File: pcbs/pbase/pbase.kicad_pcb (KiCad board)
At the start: 2 copper layers, 152.9 x 129.5 mm, 40 parts, among them J1 SD_Card, J2 Conn_01x04, J3 Conn_01x04, U1 LPCXpresso_LPC1769_revB, U2 acc_mpu9250_board, U3 GPS_EM506

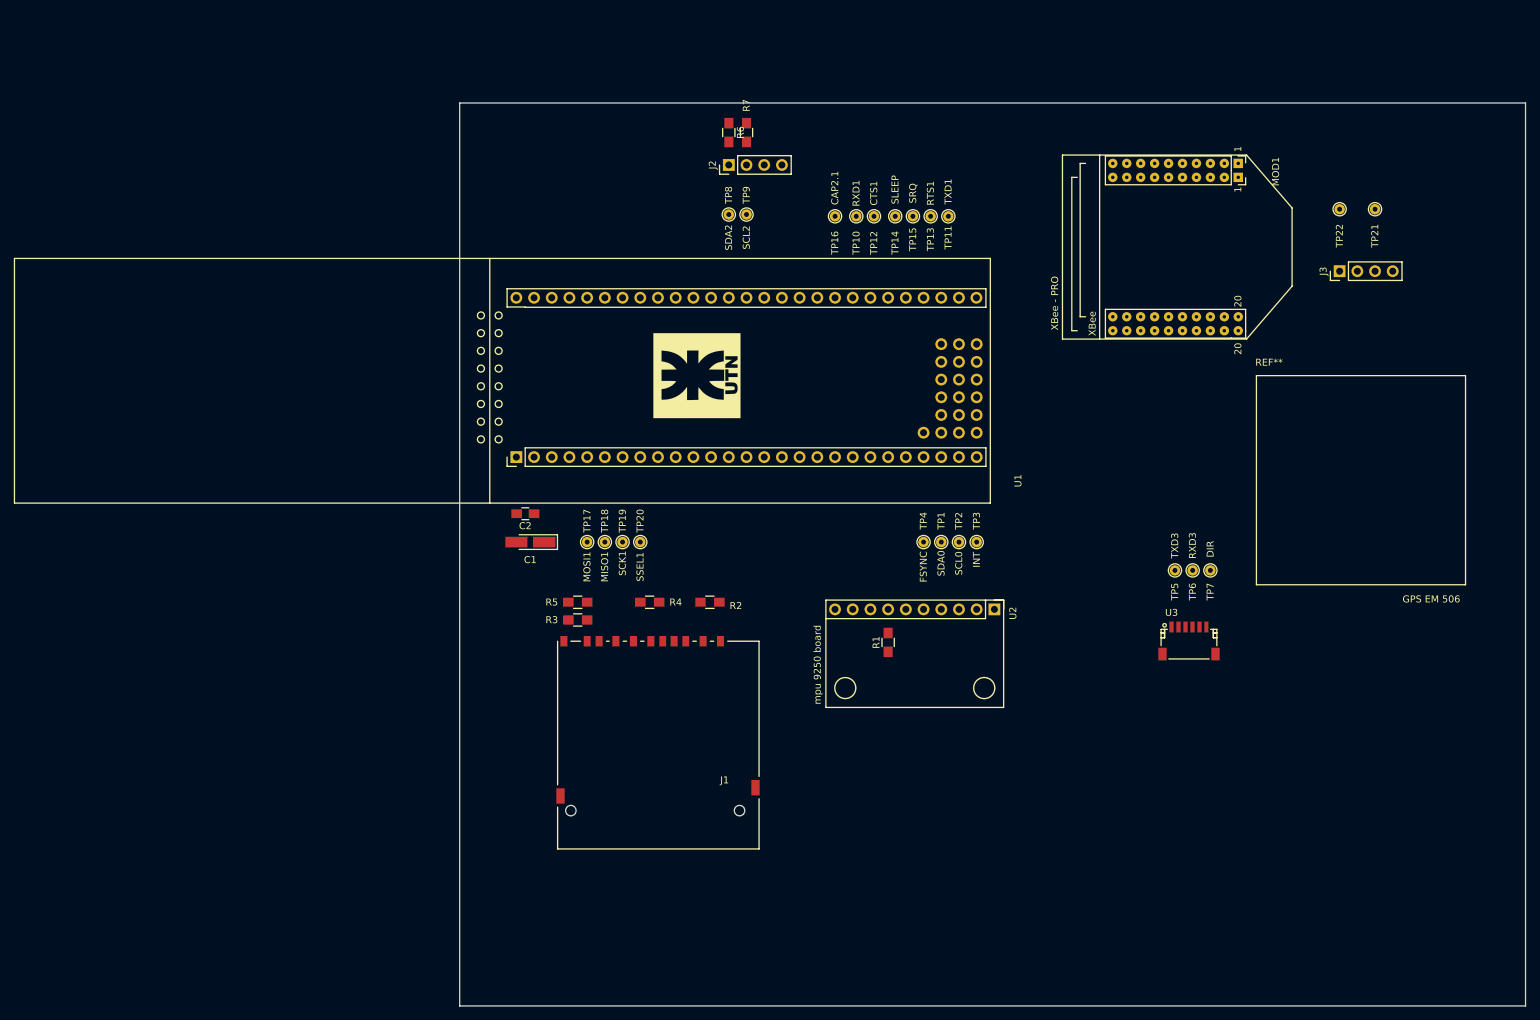
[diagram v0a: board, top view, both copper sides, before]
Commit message: PCB PLACING V1
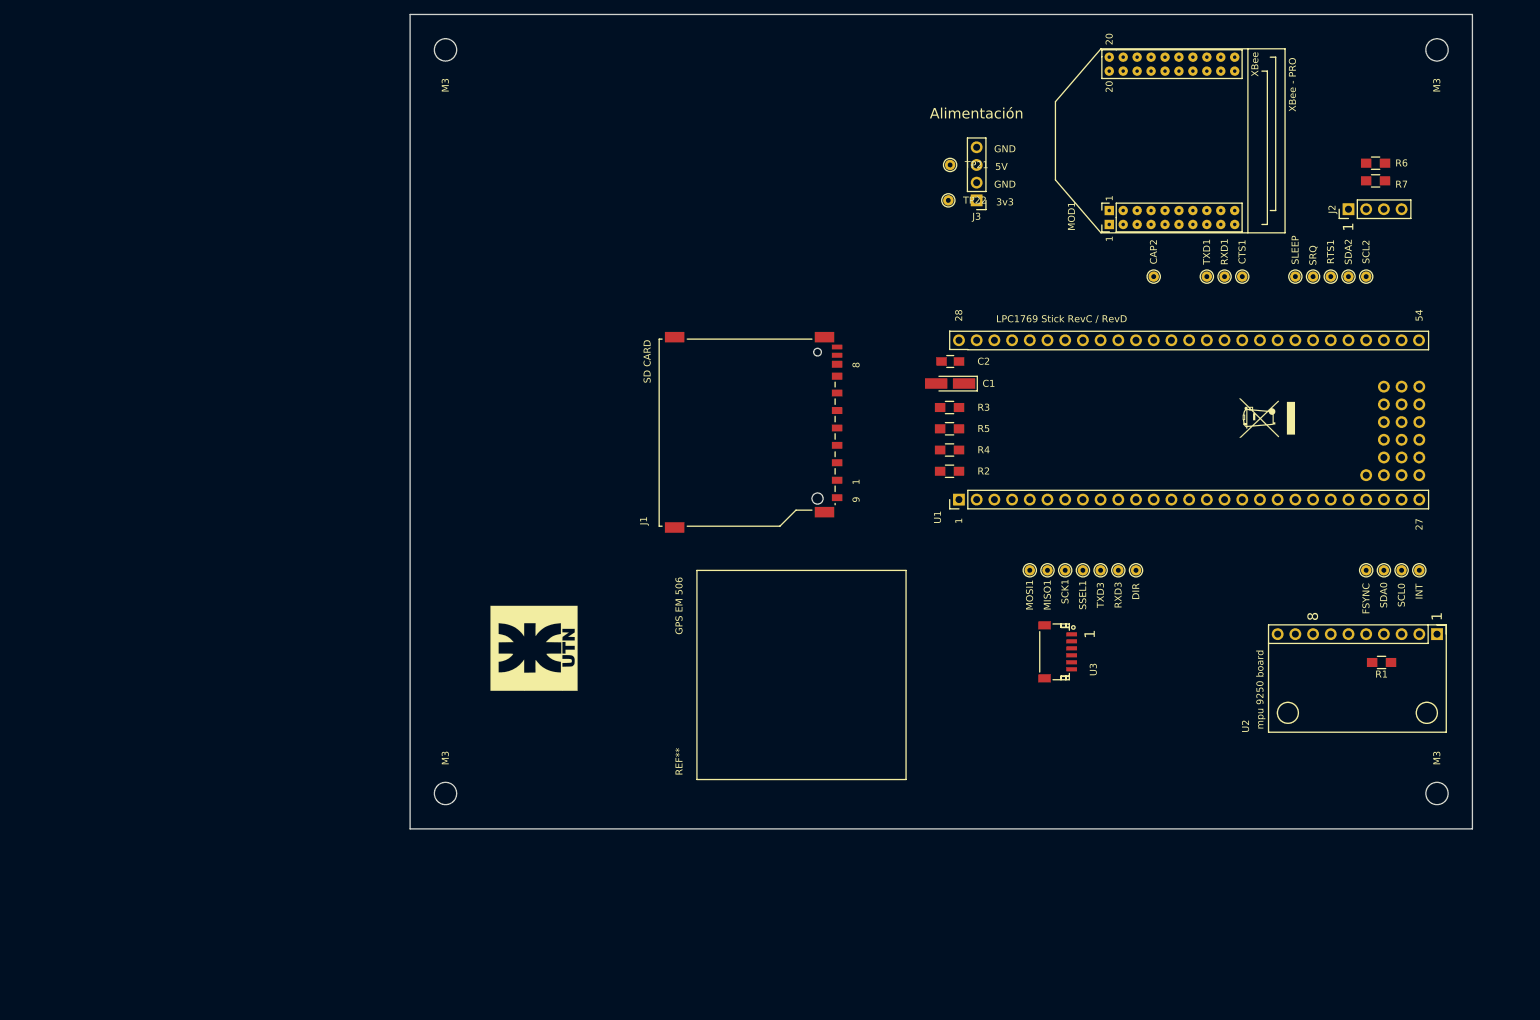
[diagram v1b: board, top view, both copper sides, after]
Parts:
- added M3: MountingHole_3.2mm_M3, Mounting_Holes:MountingHole_3.2mm_M3, F.Cu at (228.6, 30.5)
- added M3: MountingHole_3.2mm_M3, Mounting_Holes:MountingHole_3.2mm_M3, F.Cu at (228.6, 137.2)
- added M3: MountingHole_3.2mm_M3, Mounting_Holes:MountingHole_3.2mm_M3, F.Cu at (86.4, 137.2)
- added M3: MountingHole_3.2mm_M3, Mounting_Holes:MountingHole_3.2mm_M3, F.Cu at (86.4, 30.5)
- added REF***: WEEE-Logo_5.6x8mm_SilkScreen, Symbols:WEEE-Logo_5.6x8mm_SilkScreen, F.Cu at (204.2, 83.3)
- J1: footprint Connectors:SD_Card_Receptacle -> footprints:SD_TE_2041021
- TP16: value CAP2.1 -> CAP2
- moved R6 92.9 mm to (219.8, 46.7), turned to 180 degrees
- moved R7 90.5 mm to (219.8, 49.3), turned to 180 degrees
- moved TP8 89.3 mm to (215.9, 63.0)
- moved TP9 89.3 mm to (218.4, 63.0)
- moved J2 89.1 mm to (215.9, 53.3)
- moved REF** 85.0 mm to (122.4, 105.2)
- moved R1 70.8 mm to (220.6, 118.4), turned to 180 degrees
- moved C2 64.8 mm to (158.8, 75.2)
- moved C1 64.4 mm to (158.8, 78.4)
- moved U1 63.8 mm to (160.0, 95.0)
- moved TP20 63.6 mm to (177.8, 105.1)
- moved TP1 63.6 mm to (221.0, 105.1)
- moved TP17 63.6 mm to (170.2, 105.1)
- moved TP18 63.6 mm to (172.7, 105.1)
- moved TP2 63.6 mm to (223.5, 105.1)
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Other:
- board size 152.9 x 129.5 mm -> 152.4 x 116.8 mm
- board text added: "1"
- board text added: "27"
- board text added: "28"
- board text added: "3v3"
- board text added: "54"
- board text added: "5V"
- board text added: "8"
- board text added: "9"
- board text added: "Alimentación"
- board text added: "GND"
- board text added: "LPC1769 Stick RevC / RevD"
- board text added: "MODULO CARGADOR DE BATERIA"
- board text added: "SD CARD"
- board text added: "TENGO QUE LLEGAR A 10 POR 12 CM"
